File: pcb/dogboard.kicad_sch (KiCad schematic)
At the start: 29 parts, among them J1 Barrel_Jack_Switch_Pin3Ring, J2 qtpy1, J3 Conn_01x02_Male, Q1 MMBT3904, Q2 MMBT3904, SW1 SW_Push, U1 LD1117S50TR_SOT223, U2 LM555xN

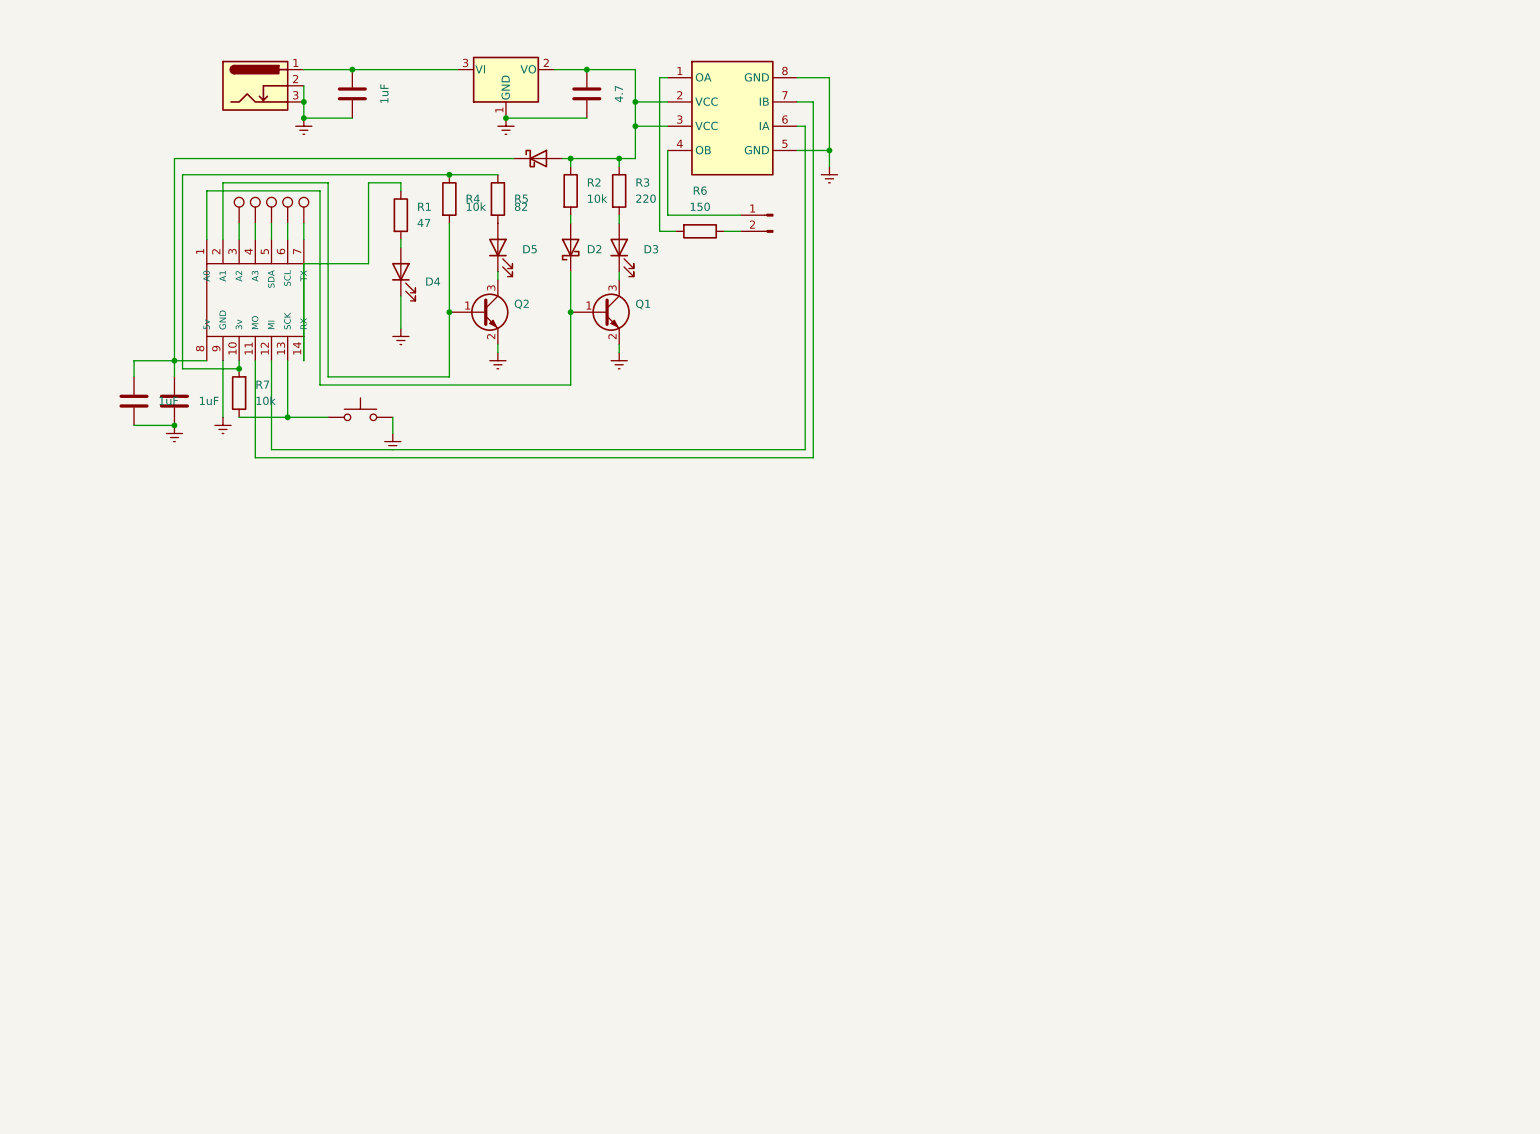
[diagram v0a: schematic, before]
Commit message: pcb refactor
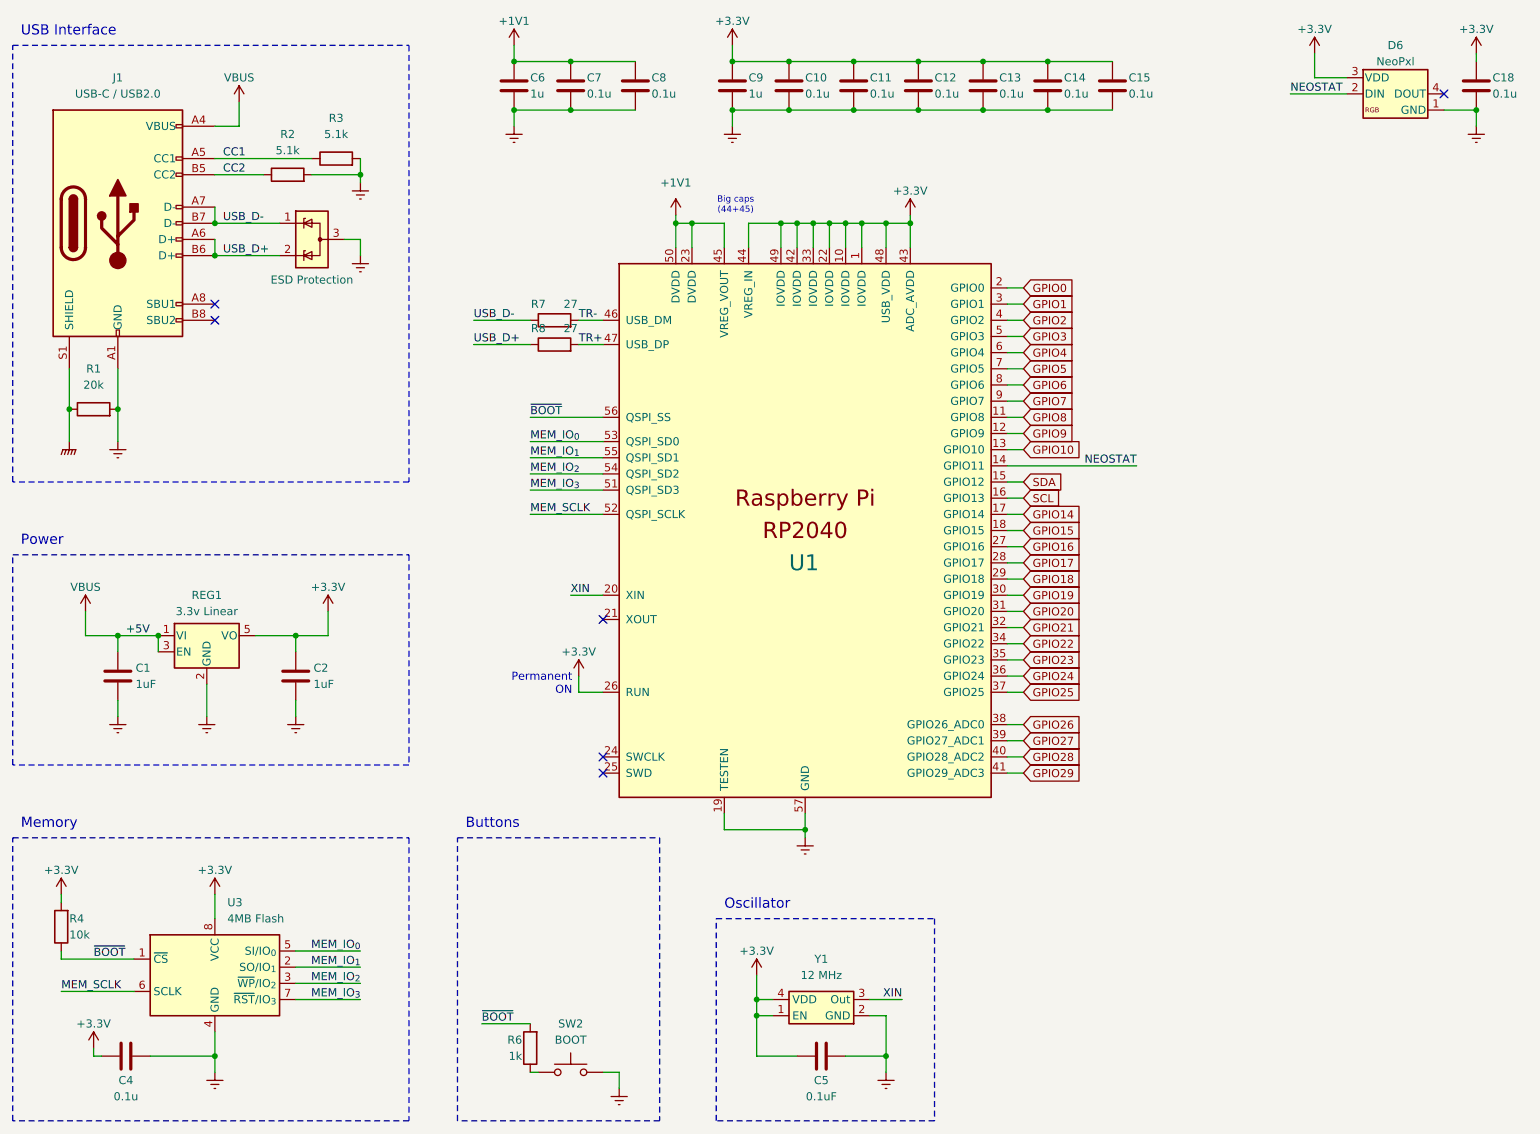
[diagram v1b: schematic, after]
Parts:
- removed C1, C3, C4: 1uF, Capacitor_SMD:C_1206_3216Metric_Pad1.33x1.80mm_HandSolder, symbol Device:C
- removed C2: 4.7, Capacitor_SMD:C_1206_3216Metric_Pad1.33x1.80mm_HandSolder, symbol Device:C
- removed D1: SB130, Diode_THT:D_DO-41_SOD81_P10.16mm_Horizontal, symbol Diode:SB130
- removed D2: D_Schottky, Diode_SMD:D_1206_3216Metric_Pad1.42x1.75mm_HandSolder, symbol Device:D_Schottky
- removed D3, D4, D5: LED, LED_SMD:LED_1206_3216Metric_Pad1.42x1.75mm_HandSolder, symbol Device:LED
- removed J1: Barrel_Jack_Switch_Pin3Ring, Connector_BarrelJack:BarrelJack_CUI_PJ-102AH_Horizontal, symbol Connector:Barrel_Jack_Switch_Pin3Ring
- removed J2: qtpy1, Module:qtpy1_reverse, symbol Device:qtpy1
- removed J3: Conn_01x02_Male, Connector_JST:JST_PH_S2B-PH-K_1x02_P2.00mm_Horizontal, symbol Connector:Conn_01x02_Male
- removed Q1, Q2: MMBT3904, Package_TO_SOT_SMD:SOT-23, symbol Transistor_BJT:MMBT3904
- removed R1: 47, Resistor_SMD:R_0805_2012Metric_Pad1.20x1.40mm_HandSolder, symbol Device:R
- removed R2, R4, R7: 10k, Resistor_SMD:R_0805_2012Metric_Pad1.20x1.40mm_HandSolder, symbol Device:R
- removed R3: 220, Resistor_SMD:R_0805_2012Metric_Pad1.20x1.40mm_HandSolder, symbol Device:R
- removed R5: 82, Resistor_SMD:R_0805_2012Metric_Pad1.20x1.40mm_HandSolder, symbol Device:R
- removed R6: 150, Resistor_SMD:R_1206_3216Metric_Pad1.30x1.75mm_HandSolder, symbol Device:R
- removed SW1: SW_Push, Button_Switch_THT:SW_PUSH-12mm, symbol Switch:SW_Push
- removed TP3, TP4, TP5, TP6, TP7: TestPoint, TestPoint:TestPoint_Pad_D1.5mm, symbol Connector:TestPoint
- removed U1: LD1117S50TR_SOT223, Package_TO_SOT_SMD:SOT-223-3_TabPin2, symbol Regulator_Linear:LD1117S50TR_SOT223
- removed U2: LM555xN, Package_DIP:DIP-8_W7.62mm, symbol Timer:LM555xN
- added C1, C2: 1uF, _custom:CAP_0805_HandSolder, symbol _custom:CAP_Standard
- added C10, C11, C12, C13, C14, C15, C18, C7, C8: 0.1u, _custom:CAP_0402_HandSolder, symbol _custom:CAP_Standard
- added C4: 0.1u, _custom:CAP_0603_HandSolder, symbol _custom:CAP_Standard
- added C5: 0.1uF, _custom:CAP_0603_HandSolder, symbol _custom:CAP_Standard
- added C6, C9: 1u, _custom:CAP_0603_HandSolder, symbol _custom:CAP_Standard
- added D1: ESD Protection, _custom:tvs_USB2_SOT-723, symbol _custom:TVS_USB_ESD_Protection
- added D6: NeoPxl, _custom:LED_NeoPixel_0606, symbol _custom:LED_NeoPixel
- added J1: USB-C / USB2.0, _custom:USB_C_Receptacle_SMD_GCT, symbol _custom:USB_C_Receptacle_USB2.0_Only
- added R1: 20k, _custom:R_0805_HandSolder, symbol _custom:Resistor_Standard
- added R2, R3: 5.1k, _custom:R_0603_HandSolder, symbol _custom:Resistor_Standard
- added R4: 10k, _custom:R_0805_HandSolder, symbol _custom:Resistor_Standard
- added R6: 1k, _custom:R_0805_HandSolder, symbol _custom:Resistor_Standard
- added R7, R8: 27, _custom:R_0402_HandSolder, symbol _custom:Resistor_Standard
- added REG1: 3.3v Linear, _custom:reg_SMD_SOT-25, symbol _custom:Regulator_SOT-25
- added SW2: BOOT, _custom:button_SMD_PTS810, symbol _custom:SW_Button_Push
- added U1: RP2040, _custom:RP2040_QFN-56, symbol _custom:RP2040
- added U3: 4MB Flash, _custom:flash_SMD_XSON-8_4x4mm, symbol _custom:Flash_Standard
- added Y1: 12 MHz, _custom:XO_Osc_4-SMD_3.2x2.5, symbol _custom:Oscillator_4pin
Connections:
- net GNDREF: now also C1.1, C10.2, C11.2, C12.2, C13.2, C14.2, C15.2, C18.2, C2.1, C4.1, C5.2, C6.2, C7.2, C8.2, C9.2, D1.3 (A), D6.1 (GND), J1.A1 (GND), J1.A12 (GND), J1.B1 (GND), J1.B12 (GND), R1.2, R2.2, R3.2, REG1.2 (GND), SW2.2, U1.19 (TESTEN), U1.57 (GND), U3.4 (GND), Y1.2 (GND)
- new net: R6.1, SW2.1
- new net +1V1: C6.1, C7.1, C8.1, U1.23 (DVDD), U1.45 (VREG_VOUT), U1.50 (DVDD)
- new net +3.3V: C10.1, C11.1, C12.1, C13.1, C14.1, C15.1, C18.1, C2.2, C4.2, C5.1, C9.1, D6.3 (VDD), R4.2, REG1.5 (VO), U1.1 (IOVDD), U1.10 (IOVDD), U1.22 (IOVDD), U1.26 (RUN), U1.33 (IOVDD), U1.42 (IOVDD), U1.43 (ADC_AVDD), U1.44 (VREG_IN), U1.48 (USB_VDD), U1.49 (IOVDD), U3.8 (VCC), Y1.1 (EN), Y1.4 (VDD)
- new net CC1: J1.A5 (CC1), R3.1
- new net CC2: J1.B5 (CC2), R2.1
- new net GNDPWR: J1.S1 (SHIELD), R1.1
- new net GPIO0: U1.2 (GPIO0)
- new net GPIO1: U1.3 (GPIO1)
- new net GPIO10: U1.13 (GPIO10)
- new net GPIO14: U1.17 (GPIO14)
- new net GPIO15: U1.18 (GPIO15)
- new net GPIO16: U1.27 (GPIO16)
- new net GPIO17: U1.28 (GPIO17)
- new net GPIO18: U1.29 (GPIO18)
- new net GPIO19: U1.30 (GPIO19)
- new net GPIO2: U1.4 (GPIO2)
- new net GPIO20: U1.31 (GPIO20)
- new net GPIO21: U1.32 (GPIO21)
- new net GPIO22: U1.34 (GPIO22)
- new net GPIO23: U1.35 (GPIO23)
- new net GPIO24: U1.36 (GPIO24)
- new net GPIO25: U1.37 (GPIO25)
- new net GPIO26: U1.38 (GPIO26_ADC0)
- new net GPIO27: U1.39 (GPIO27_ADC1)
- new net GPIO28: U1.40 (GPIO28_ADC2)
- new net GPIO29: U1.41 (GPIO29_ADC3)
- new net GPIO3: U1.5 (GPIO3)
- new net GPIO4: U1.6 (GPIO4)
- new net GPIO5: U1.7 (GPIO5)
- new net GPIO6: U1.8 (GPIO6)
- new net GPIO7: U1.9 (GPIO7)
- new net GPIO8: U1.11 (GPIO8)
- new net GPIO9: U1.12 (GPIO9)
- new net MEM_IO_{0}: U1.53 (QSPI_SD0), U3.5 (SI/IO_{0})
- new net MEM_IO_{1}: U1.55 (QSPI_SD1), U3.2 (SO/IO_{1})
- new net MEM_IO_{2}: U1.54 (QSPI_SD2), U3.3 (~{WP}/IO_{2})
- new net MEM_IO_{3}: U1.51 (QSPI_SD3), U3.7 (~{RST}/IO_{3})
- new net MEM_SCLK: U1.52 (QSPI_SCLK), U3.6 (SCLK)
- new net NEOSTAT: D6.2 (DIN), U1.14 (GPIO11)
- new net SCL: U1.16 (GPIO13)
- new net SDA: U1.15 (GPIO12)
- new net TR+: R8.2, U1.47 (USB_DP)
- new net TR-: R7.2, U1.46 (USB_DM)
- new net USB_D+: D1.2 (K), J1.A6 (D+), J1.B6 (D+), R8.1
- new net USB_D-: D1.1 (K), J1.A7 (D-), J1.B7 (D-), R7.1
- new net VBUS: C1.2, J1.A4 (VBUS), J1.A9 (VBUS), J1.B4 (VBUS), J1.B9 (VBUS), REG1.1 (VI), REG1.3 (EN)
- new net XIN: U1.20 (XIN), Y1.3 (Out)
- new net ~{BOOT}: R4.1, R6.2, U1.56 (QSPI_SS), U3.1 (~{CS})
- no-connect marks 0 -> 6
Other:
- note added: "Big caps (44+45)"
- note added: "Buttons"
- note added: "Memory"
- note added: "Oscillator"
- note added: "Permanent ON"
- note added: "Power"
- note added: "USB Interface"
